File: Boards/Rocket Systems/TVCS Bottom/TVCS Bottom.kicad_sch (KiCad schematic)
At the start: 102 parts, among them IC1 NSVT30010MXV6T1G, IC2 NSVT30010MXV6T1G, J1 Conn_01x01_Socket, J10 Conn_01x01_Socket, J11 Conn_01x01_Socket, J12 Conn_01x01_Socket, J2 1190297, J3 XT30UPB-M, J4 XT30UPB-M, J5 1190298, J6 XT30UPB-M, J8 Conn_01x01_Socket, J9 Conn_01x01_Socket, Q1 2N7002H6327XTSA2, U1 MAX31856MUD+T, U10 MAX31856MUD+T, U11 IRLZ44NPBF, U12 IRLZ44NPBF, U13 LM61460AASQRJRRQ1, U14 ADS1114IRUGR, U17 MAX485CSA+T, U3 MAX31856MUD+T, U4 PCA9306DP_118, U5 MCP9808T-E/MC, U9 LM61460AASQRJRRQ1

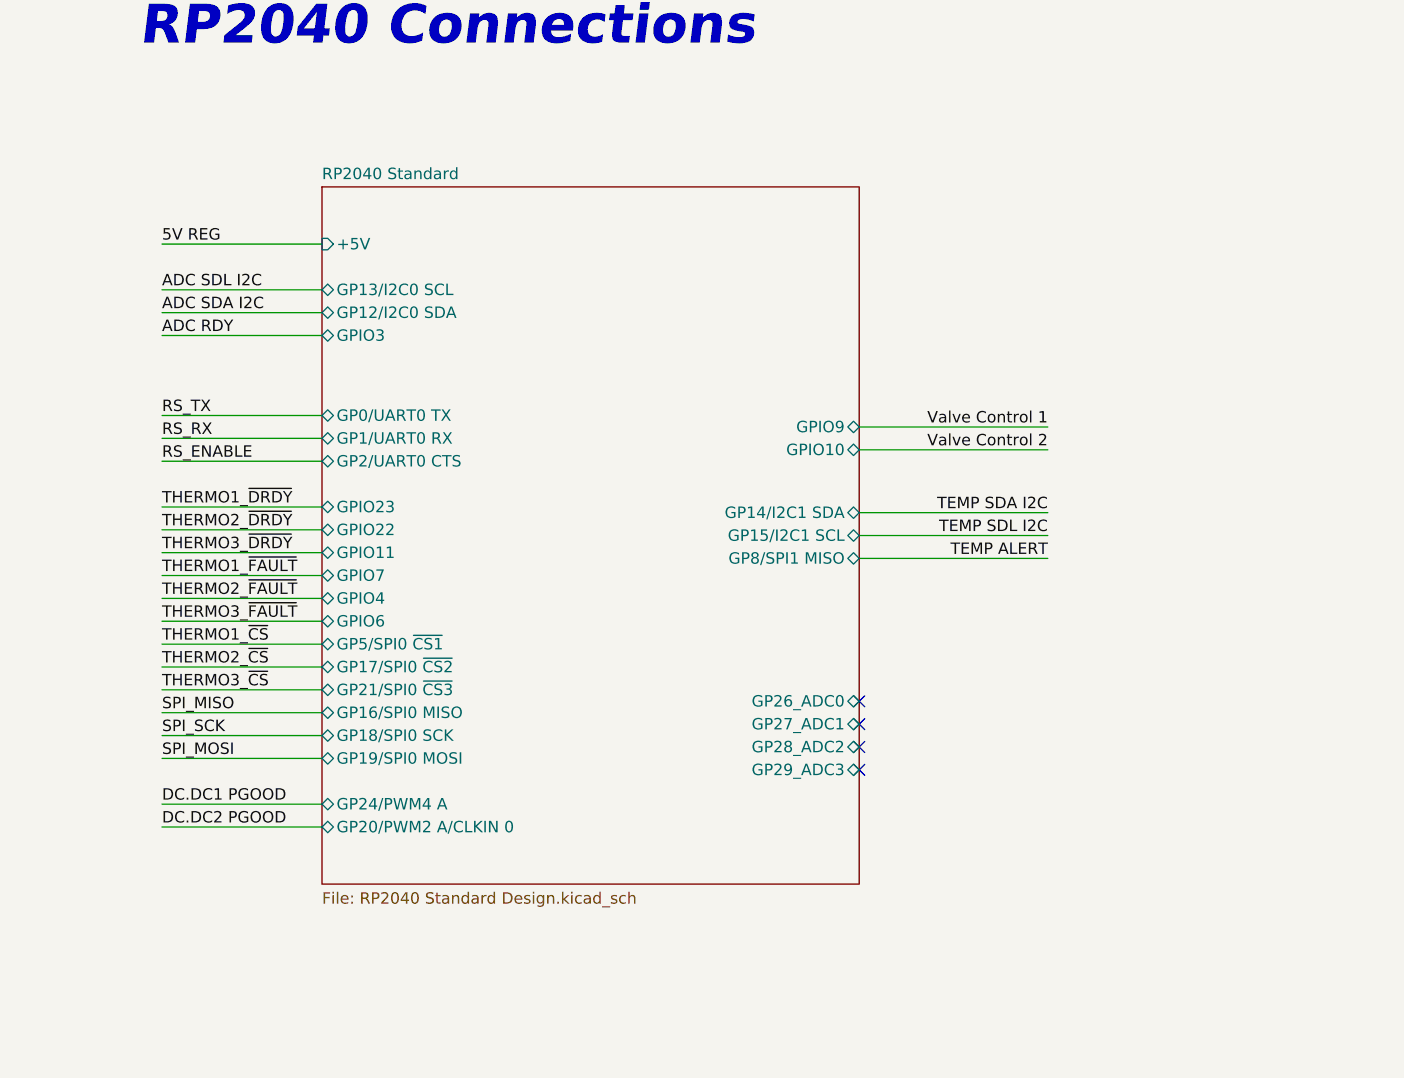
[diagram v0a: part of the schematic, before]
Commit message: Mais Sockets Pico
TVCS Top, Bottom and Fill and G&F COMMS
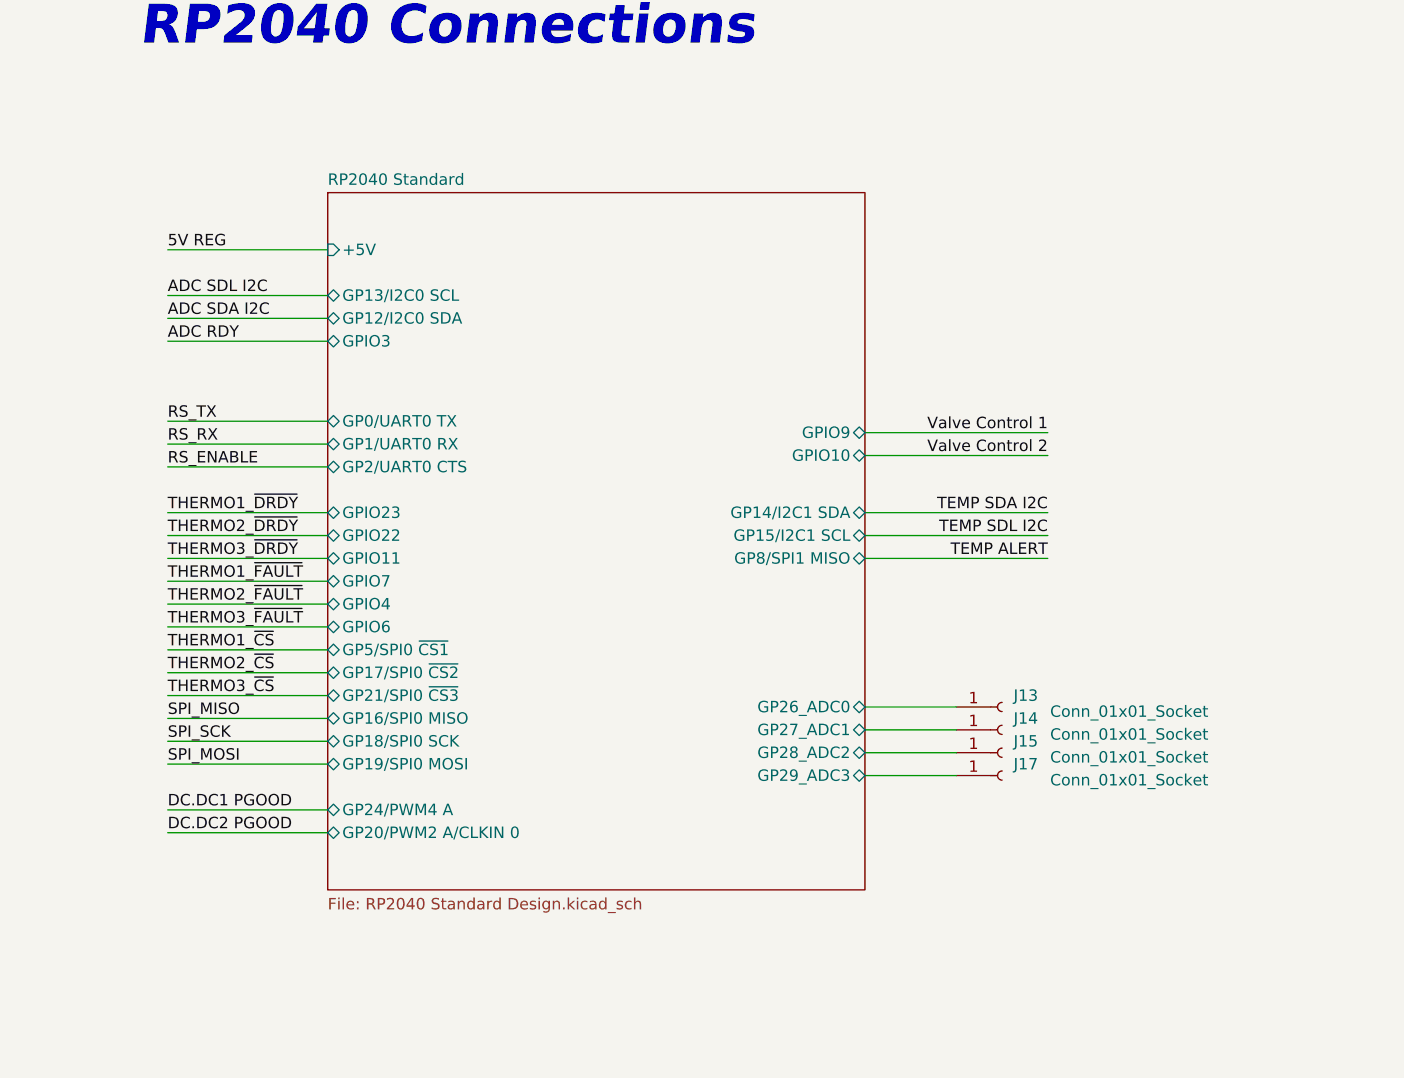
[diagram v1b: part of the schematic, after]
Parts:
- added J13, J14, J15, J17: Conn_01x01_Socket, Pico_Conn1x1:Pico_01pin, symbol Connector:Conn_01x01_Socket
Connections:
- net RP2040 Standard/GP26_ADC0: now also J13.1 (Pin_1)
- net RP2040 Standard/GP27_ADC1: now also J14.1 (Pin_1)
- net RP2040 Standard/GP28_ADC2: now also J15.1 (Pin_1)
- net RP2040 Standard/GP29_ADC3: now also J17.1 (Pin_1)
- no-connect marks 4 -> 0
